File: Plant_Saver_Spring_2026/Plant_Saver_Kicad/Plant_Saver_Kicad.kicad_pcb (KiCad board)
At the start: 2 copper layers, 111 parts, among them J10 DM3D-SF, J11 Test, J2 SBH11-PBPC-D05-ST-BK, J3 SM04B-SRSS-TB, J5 Conn_01x02_Pin, J6 Conn_01x06_Socket, J7 S3B-PH-K-S, J8 54-00284, J9 1.25mm, Q1 G09P02L, Q10 G09P02L, Q11 ISP12DP06NMXTSA1, Q12 G09P02L, Q2 G09P02L, Q3 ISP12DP06NMXTSA1, Q4 G09P02L, Q5 G09P02L, Q6 G09P02L, Q7 G09P02L, Q8 G09P02L, Q9 G09P02L, SW1 Reset, SW2 25336NA, SW3 Boot, SW4 SA72SB0, U1 CDBA140SL-HF, U10 DW03C, U11 CDBA140SL-HF, U12 LP38511TJ-ADJ/NOPB, U13 MCP73833-xxx-UN, U14 MCP6234, U15 MCP73833-xxx-UN, U16 MCP6547T_I_MS, U2 CDBA140SL-HF, U3 CDBA140SL-HF, U4 CDBA140SL-HF, U5 ESP32-WROOM-32E-N16, U9 CDBA140SL-HF

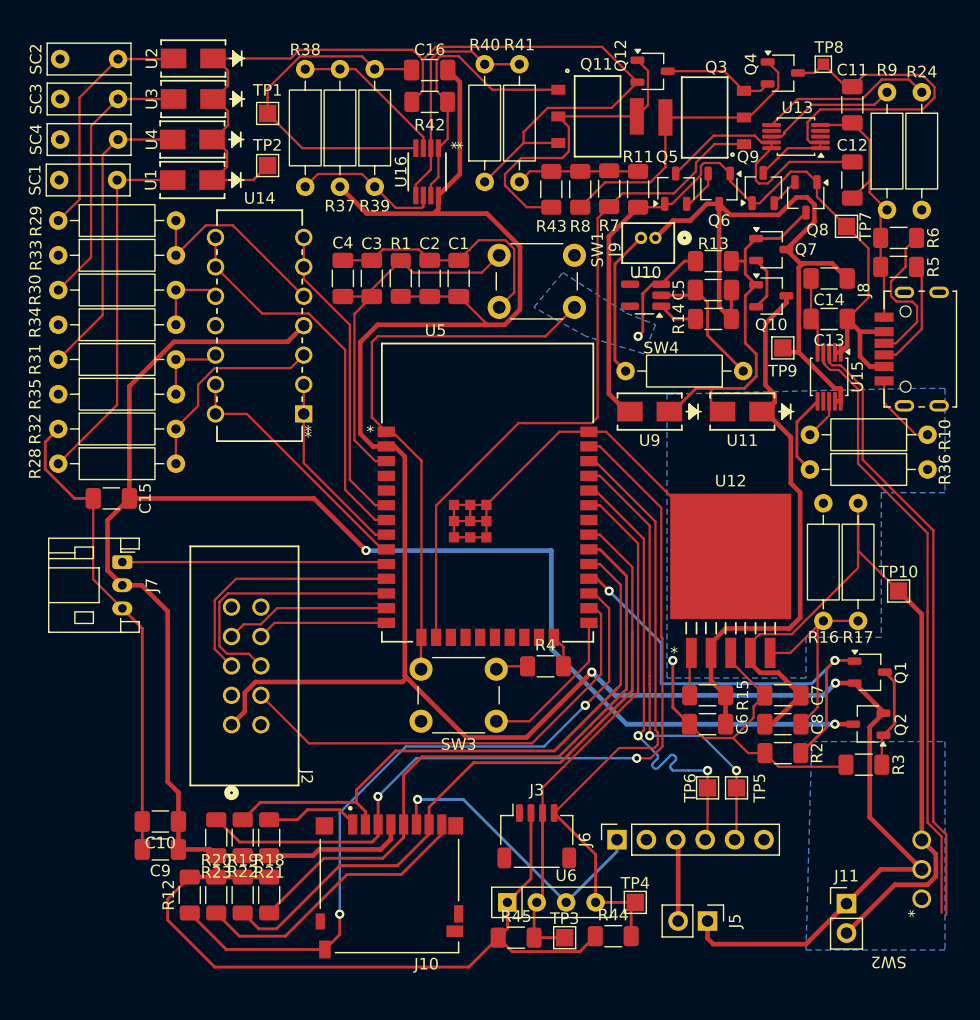
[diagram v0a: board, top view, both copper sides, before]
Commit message: PCB Pre-Check complete
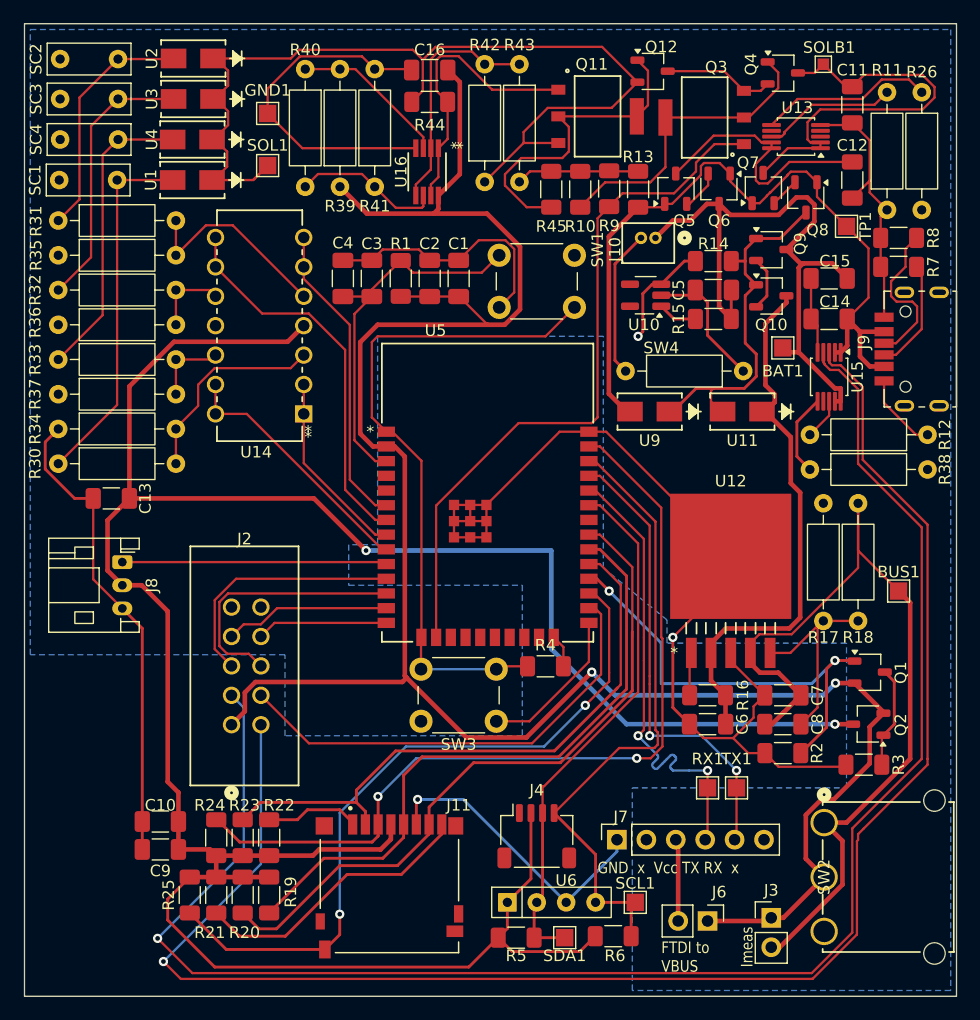
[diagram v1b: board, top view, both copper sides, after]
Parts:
- removed the J11 at (98.0, 144.0)
- added J3: Test, Connector_PinHeader_2.54mm:PinHeader_1x02_P2.54mm_Vertical, F.Cu at (91.5, 145.2)
- SW2: value 25336NA -> 1101M2S3AQE2; footprint 25336NA:SWITCH_25336NA_APM -> 1101M2S3AQE2:SPDT-1101M2_CNK
- moved SW2 10.7 mm to (96.1, 137.0)
- renumbered TP9 to BAT1, TP10 to BUS1, C15 to C13, C13 to C14, C14 to C15, TP1 to GND1, J9 to J10, J10 to J11, J3 to J4, J5 to J6, J6 to J7, J7 to J8, J8 to J9, R8 to R10, R9 to R11, R10 to R12, R11 to R13, R13 to R14, R14 to R15, R15 to R16, R16 to R17, R17 to R18, R18 to R19, R19 to R20, R20 to R21, R21 to R22, R22 to R23, R23 to R24, R12 to R25, R24 to R26, R28 to R30, R29 to R31, R30 to R32, R31 to R33, R32 to R34, R33 to R35, R34 to R36, R35 to R37, R36 to R38, R37 to R39, R38 to R40, R39 to R41, R40 to R42, R41 to R43, R42 to R44, R43 to R45, R45 to R5, R44 to R6, R5 to R7, R6 to R8, R7 to R9, TP6 to RX1, TP4 to SCL1, TP3 to SDA1, TP2 to SOL1, TP8 to SOLB1, TP7 to TP1, TP5 to TX1
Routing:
- net STAT2: track 53.1 -> 143.8 mm, vias 0 -> 1
- net STAT1: track 53.2 -> 142.8 mm, vias 0 -> 1
- net GND: track 303.2 -> 320.8 mm
- net Vbus: track 196.7 -> 187.8 mm
- net /Power_And_Charging/Vout: track 73.8 -> 77.1 mm
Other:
- board outline added: 80.5 x 84 mm
- board text added: "FTDI to VBUS"
- board text added: "GND x Vcc TX RX x"
- board text added: "Imeas"
